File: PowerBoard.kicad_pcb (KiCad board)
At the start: 2 copper layers, 21.7 x 14.5 mm, 10 parts

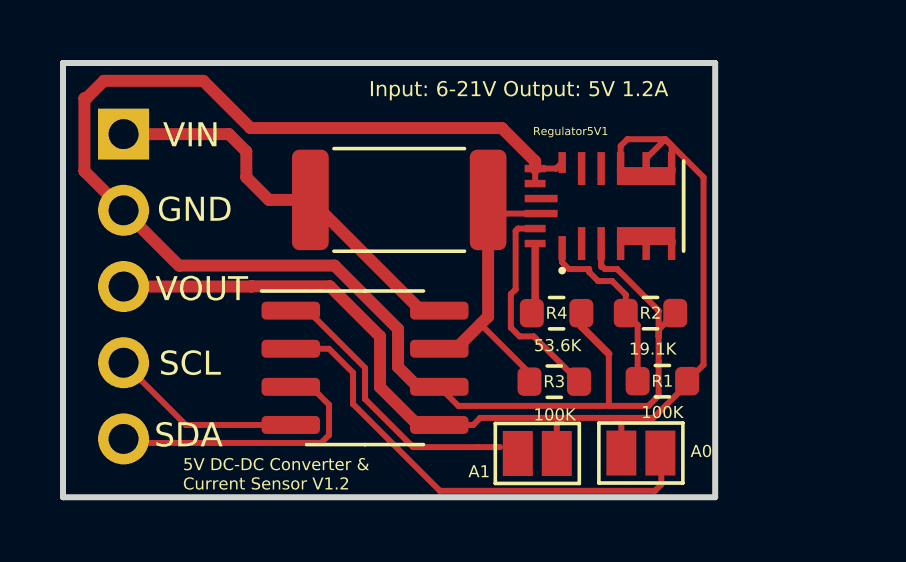
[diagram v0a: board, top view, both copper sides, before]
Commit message: update to 1.3.
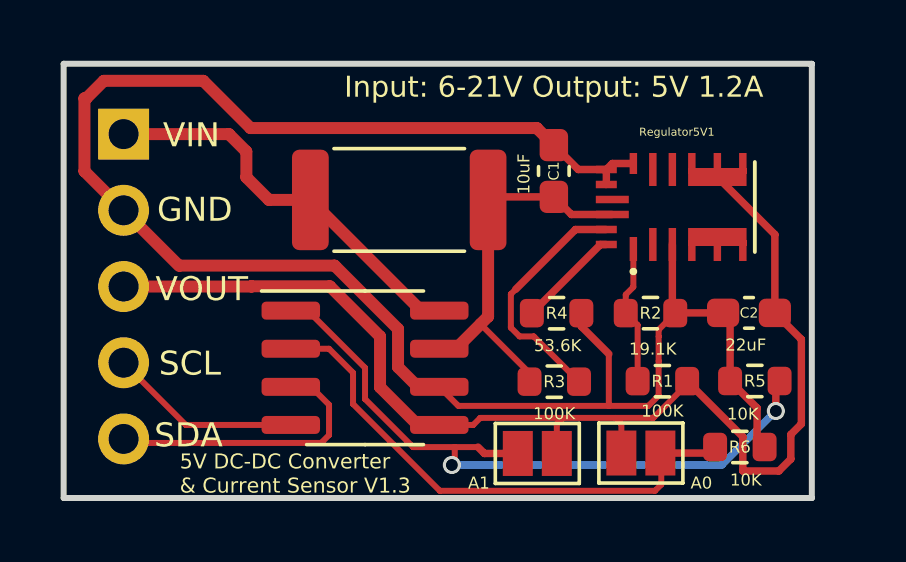
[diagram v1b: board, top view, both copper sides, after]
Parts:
- added C1: 10uF, Capacitor_SMD:C_0603_1608Metric_Pad1.08x0.95mm_HandSolder, F.Cu at (130.9, 54.4)
- added C2: 22uF, Capacitor_SMD:C_0603_1608Metric_Pad1.08x0.95mm_HandSolder, F.Cu at (137.4, 59.1)
- added R5: 10K, Resistor_SMD:R_0603_1608Metric, F.Cu at (137.6, 61.4)
- added R6: 10K, Resistor_SMD:R_0603_1608Metric, F.Cu at (137.1, 63.6)
- moved Regulator5V1 2.37 mm to (135.1, 55.6)
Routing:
- net Net-(A1-Pad1): track 9.47 -> 23.4 mm, vias 0 -> 2
- net GND: track 55.1 -> 61.4 mm
- net +5V: track 37.8 -> 41.1 mm
- net Net-(C1-Pad1): track 10.9 -> 13.3 mm
- net Net-(A0-Pad1): track 16.0 -> 17.9 mm
- net Net-(R1-Pad2): track 6.15 -> 4.67 mm
- net Net-(R3-Pad2): track 6.99 -> 8.21 mm
- net Net-(R4-Pad1): track 2.37 -> 3.43 mm
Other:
- board size 21.7 x 14.5 mm -> 24.9 x 14.5 mm
- board text added: "5V DC-DC Converter & Current Sensor V1.3"
- board text removed: "5V Buck Converter & Current Sensor V1.2 The default I2C address for this device is 0x40. You can adjust the address of the device by shorting jumpers A0 and A1. See the table in the INA219 datasheet for more details. I2C Address A0 A1 0x40 Open Open 0x41 Open Closed 0x44 Closed Open It is possible to adjust the voltage output. This can be achieved by swapping out the resistors as defined in the f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"
- board text removed: "5V DC-DC Converter & Current Sensor V1.2"
